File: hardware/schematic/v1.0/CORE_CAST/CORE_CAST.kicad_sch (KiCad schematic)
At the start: 86 parts, among them J1 Conn_01x06_Socket, J10 USB_C_Receptacle_USB2.0_16P, J11 Conn_01x06_Socket, J12 Conn_Coaxial, J13 Conn_01x04_Socket, J14 Conn_01x03_Socket, J15 Conn_01x05_Socket, J16 Conn_01x04_Socket, J17 Conn_Coaxial, J18 Conn_Coaxial, J19 Conn_Coaxial, J2 Conn_Coaxial, J20 Conn_Coaxial, J21 Conn_Coaxial, J22 Conn_Coaxial, J23 Conn_Coaxial, J24 Conn_Coaxial, J3 Conn_Coaxial, J4 Conn_Coaxial, J5 Conn_Coaxial, J6 Conn_Coaxial, J7 Conn_Coaxial, J8 Conn_Coaxial, J9 Conn_Coaxial, M1 ZYNQ7010&7020, U1 TXS02612RTWR, U2 TPS78633, U3 SD_Card, U4 *, U5 AMS1117-1.8, U6 CH340E

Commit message: sch update
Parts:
- added J25: HDMI_A, Connector_Video:HDMI_A_Molex_208658-1001_Horizontal, symbol Connector:HDMI_A
- added U7: FPC-6P, symbol Counter:FPC-6P
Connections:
- net +3.3V: now also U7.2
- net GND: now also U7.3, U7.7 (SH), U7.8 (SH)
- new net CTP_INT: U7.4
- new net CTP_RST: U7.1
- new net CTP_SCL: U7.6
- new net CTP_SDA: U7.5
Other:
- moved on the sheet: C2, C3, C4, C5, D3, D4, D5, D6, R15, R16, R17, R18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

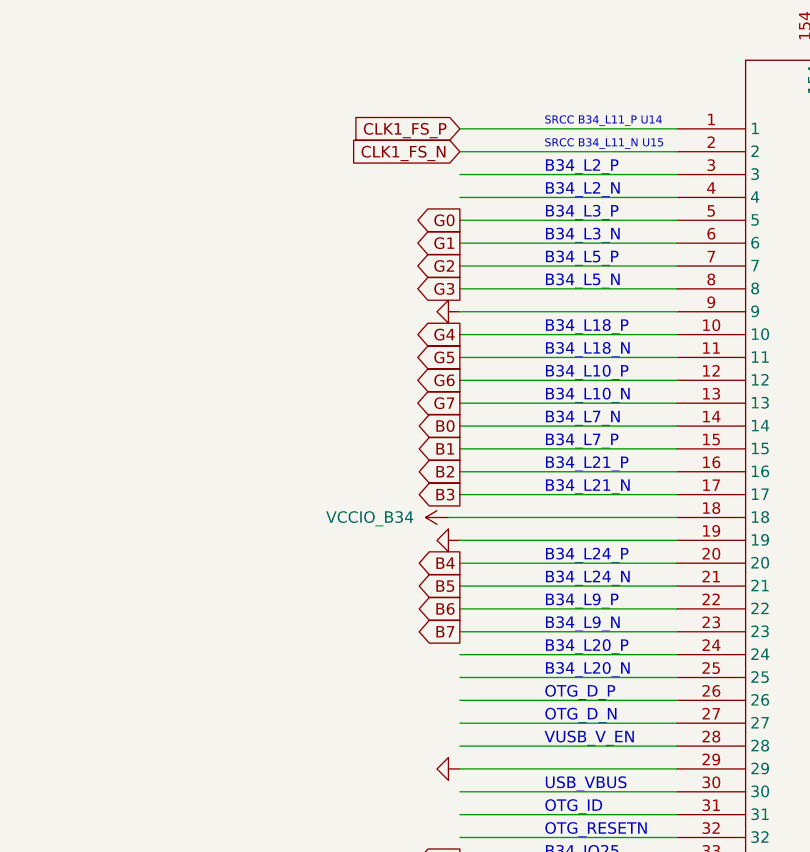
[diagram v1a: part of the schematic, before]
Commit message: sch update
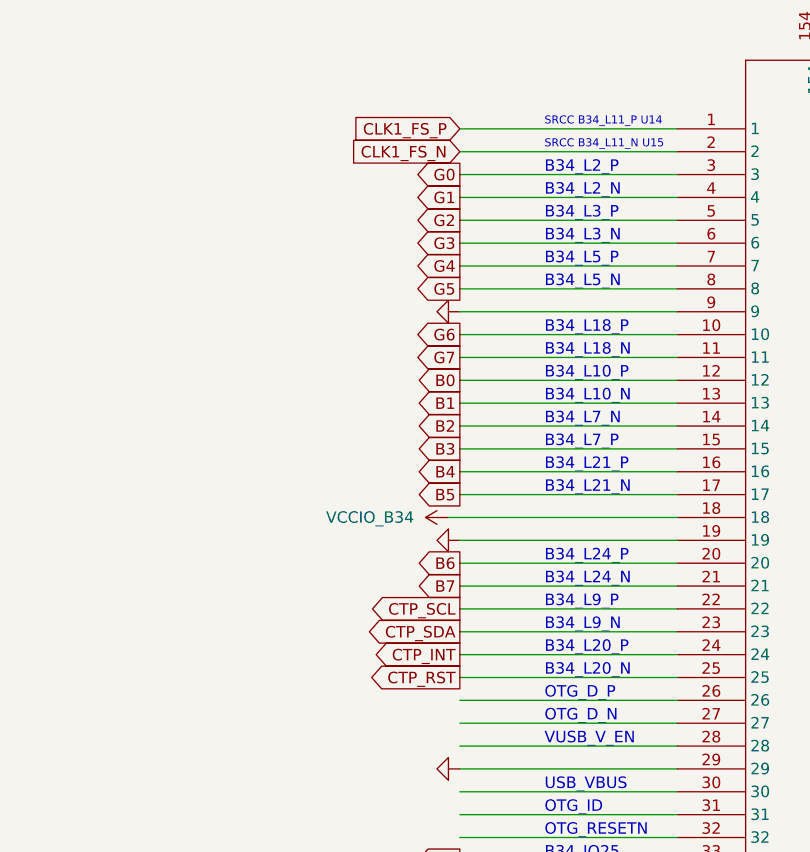
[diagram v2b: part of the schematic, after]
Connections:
- net B0: now also U4.12; no longer U4.14
- net B1: now also U4.13; no longer U4.15
- net B2: now also U4.14; no longer U4.16
- net B3: now also U4.15; no longer U4.17
- net B4: now also U4.16; no longer U4.20
- net B5: now also U4.17; no longer U4.21
- net B6: now also U4.20; no longer U4.22
- net B7: now also U4.21; no longer U4.23
- net CTP_INT: now also U4.24
- net CTP_RST: now also U4.25
- net CTP_SCL: now also U4.22
- net CTP_SDA: now also U4.23
- net G0: now also U4.3; no longer U4.5
- net G1: now also U4.4; no longer U4.6
- net G2: now also U4.5; no longer U4.7
- net G3: now also U4.6; no longer U4.8
- net G4: now also U4.7; no longer U4.10
- net G5: now also U4.8; no longer U4.11
- net G6: now also U4.10; no longer U4.12
- net G7: now also U4.11; no longer U4.13

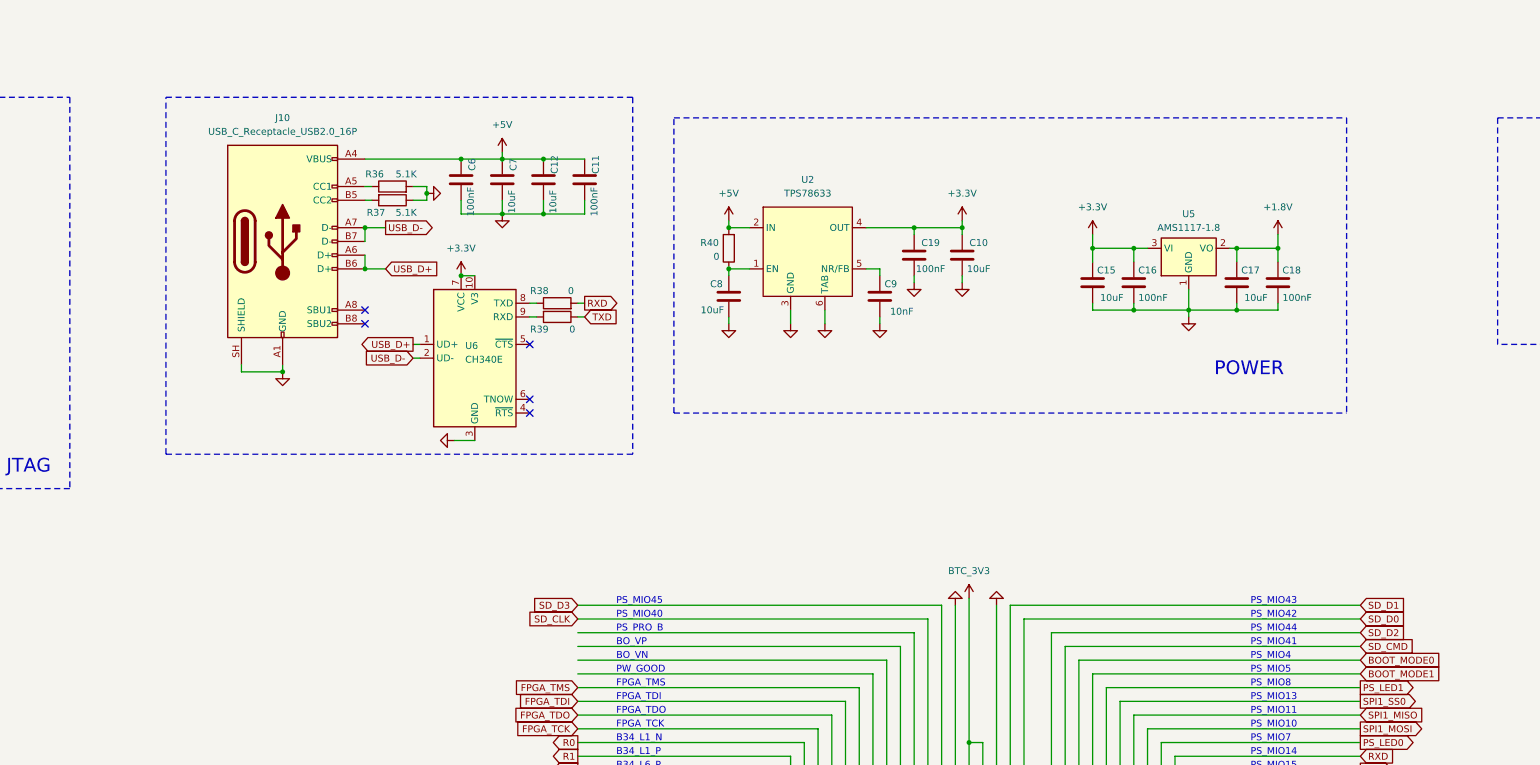
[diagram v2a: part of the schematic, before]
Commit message: sch upate
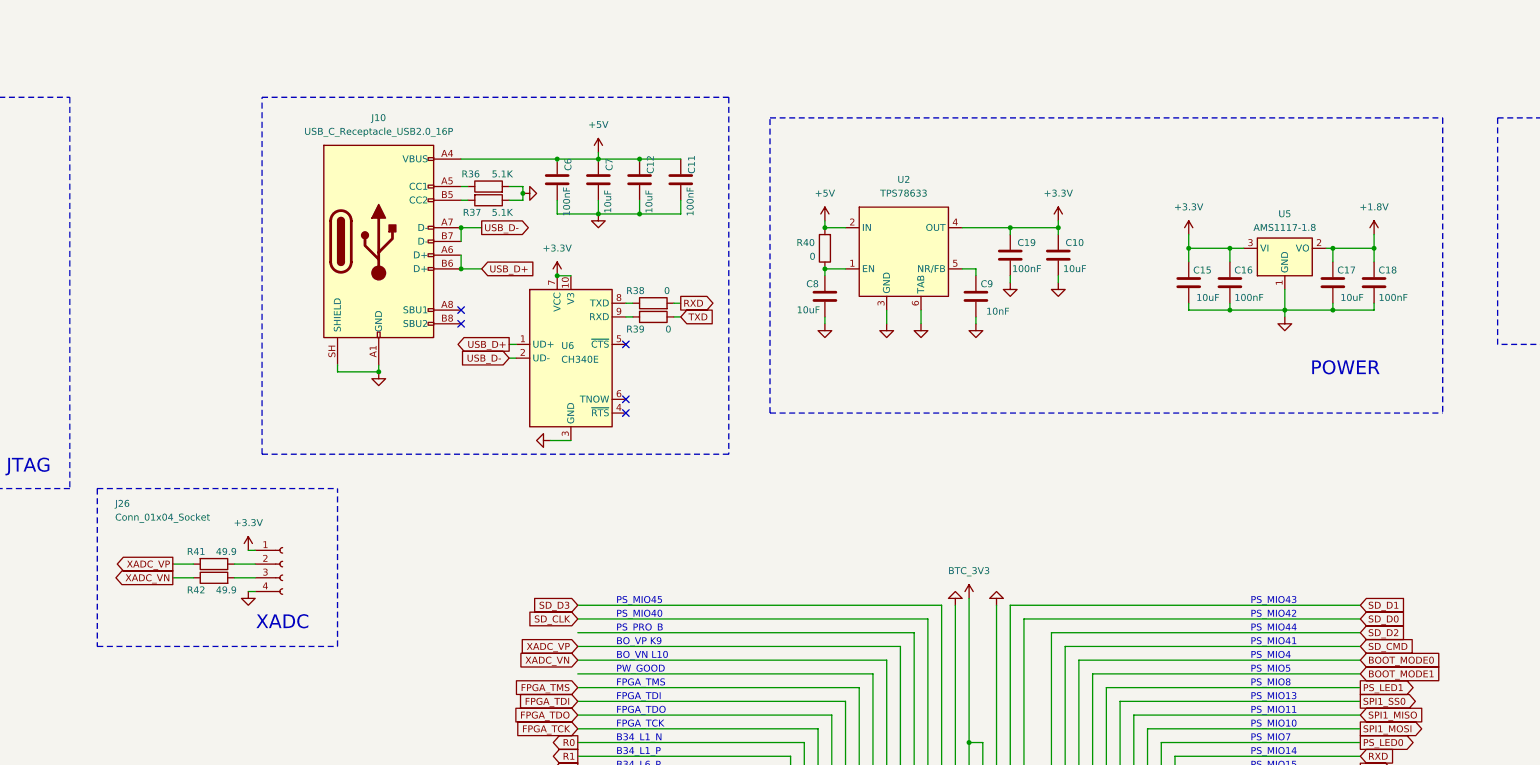
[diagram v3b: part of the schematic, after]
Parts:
- added J26: Conn_01x04_Socket, Connector_PinHeader_2.54mm:PinHeader_1x04_P2.54mm_Vertical, symbol Connector:Conn_01x04_Socket
- added R41, R42: 49.9, Resistor_SMD:R_0402_1005Metric, symbol Device:R
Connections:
- net +3.3V: now also J26.1 (Pin_1)
- net GND: now also J26.4 (Pin_4)
- net XADC_VN: now also U4.141, R42.1
- net XADC_VP: now also U4.140, R41.2
- new net: J26.2 (Pin_2), R41.1
- new net: J26.3 (Pin_3), R42.2
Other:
- note added: "BO_VN L10"
- note added: "BO_VP K9"
- note added: "XADC"
- note removed: "BO_VN"
- note removed: "BO_VP"
- moved on the sheet: C10, C11, C12, C15, C16, C17, C18, C19, C6, C7, C8, C9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

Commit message: sch update
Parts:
- added C13: 1nF, Capacitor_SMD:C_0402_1005Metric, symbol Device:C
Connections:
- net B0: now also U4.8; no longer U4.12
- net B1: now also U4.7; no longer U4.13
- net B2: now also U4.6; no longer U4.14
- net B3: now also U4.5; no longer U4.15
- net B4: now also U4.4; no longer U4.16
- net B5: now also U4.3; no longer U4.17
- net B6: now also U4.154; no longer U4.20
- net B7: now also U4.153; no longer U4.21
- net CLK: now also U4.152; no longer U4.34
- net CTP_INT: now also U4.40; no longer U4.24
- net CTP_RST: now also U4.41; no longer U4.25
- net CTP_SCL: now also U4.38; no longer U4.22
- net CTP_SDA: now also U4.39; no longer U4.23
- net DE: now also U4.148; no longer U4.33
- net DISP: now also U4.151; no longer U4.35
- net G0: now also U4.17; no longer U4.3
- net G1: now also U4.16; no longer U4.4
- net G2: now also U4.15; no longer U4.5
- net G3: now also U4.14; no longer U4.6
- net G4: now also U4.13; no longer U4.7
- net G5: now also U4.12; no longer U4.8
- net G6: now also U4.11; no longer U4.10
- net G7: now also U4.10; no longer U4.11
- net HSYNC: now also U4.150; no longer U4.36
- net I2C_SCL: no longer J14.2 (Pin_2)
- net I2C_SDA: no longer J14.1 (Pin_1)
- net R0: now also U4.35; no longer U4.147
- net R1: now also U4.34; no longer U4.148
- net R2: now also U4.25; no longer U4.149
- net R3: now also U4.24; no longer U4.150
- net R4: now also U4.23; no longer U4.151
- net R5: now also U4.22; no longer U4.152
- net R6: now also U4.21; no longer U4.153
- net R7: now also U4.20
- net SPI1_MISO: no longer J15.2 (Pin_2), U4.123
- net SPI1_MOSI: no longer J15.1 (Pin_1), U4.122
- net SPI1_SCLK: no longer J15.3 (Pin_3), U4.118
- net SPI1_SS0: no longer J15.4 (Pin_4), U4.124
- net VSYNC: now also U4.149; no longer U4.37
- net at J26.2 (Pin_2), R41.1: now also C13.1
- net at J26.3 (Pin_3), R42.2: now also C13.2
- new net PS_I2C_SCL: J14.2 (Pin_2)
- new net PS_I2C_SDA: J14.1 (Pin_1)
- new net PS_SPI1_MISO: J15.2 (Pin_2), U4.123
- new net PS_SPI1_MOSI: J15.1 (Pin_1), U4.122
- new net PS_SPI1_SCLK: J15.3 (Pin_3), U4.118
- new net PS_SPI1_SS0: J15.4 (Pin_4), U4.124
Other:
- moved on the sheet: D3, D4, D5, D6, J1, J14, J26, R41, R42, R5, R6, R7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
